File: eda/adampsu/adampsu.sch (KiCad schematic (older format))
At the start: 39 parts, among them J1 Barrel_Jack_Switch, J2 Conn_2Rows-09Pins, J3 DB9_Female, Q1 BUK7880-55A_CUX, SW1 30V 300mA Latching Switch, U1 LM27761

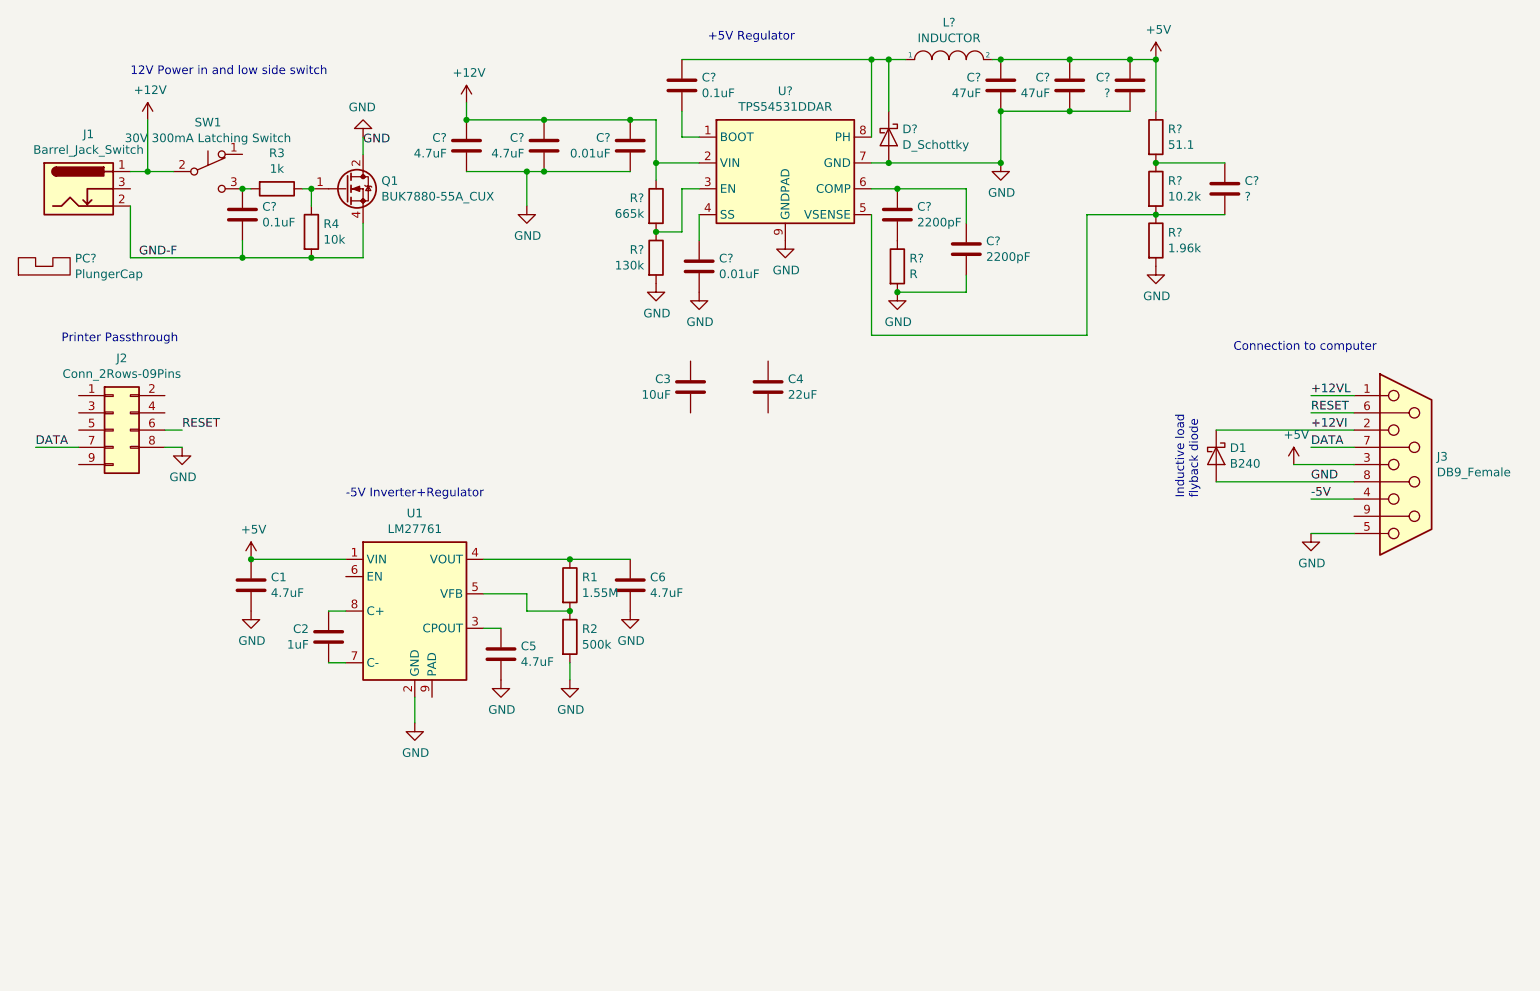
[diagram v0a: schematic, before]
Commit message: Final parts selection finished
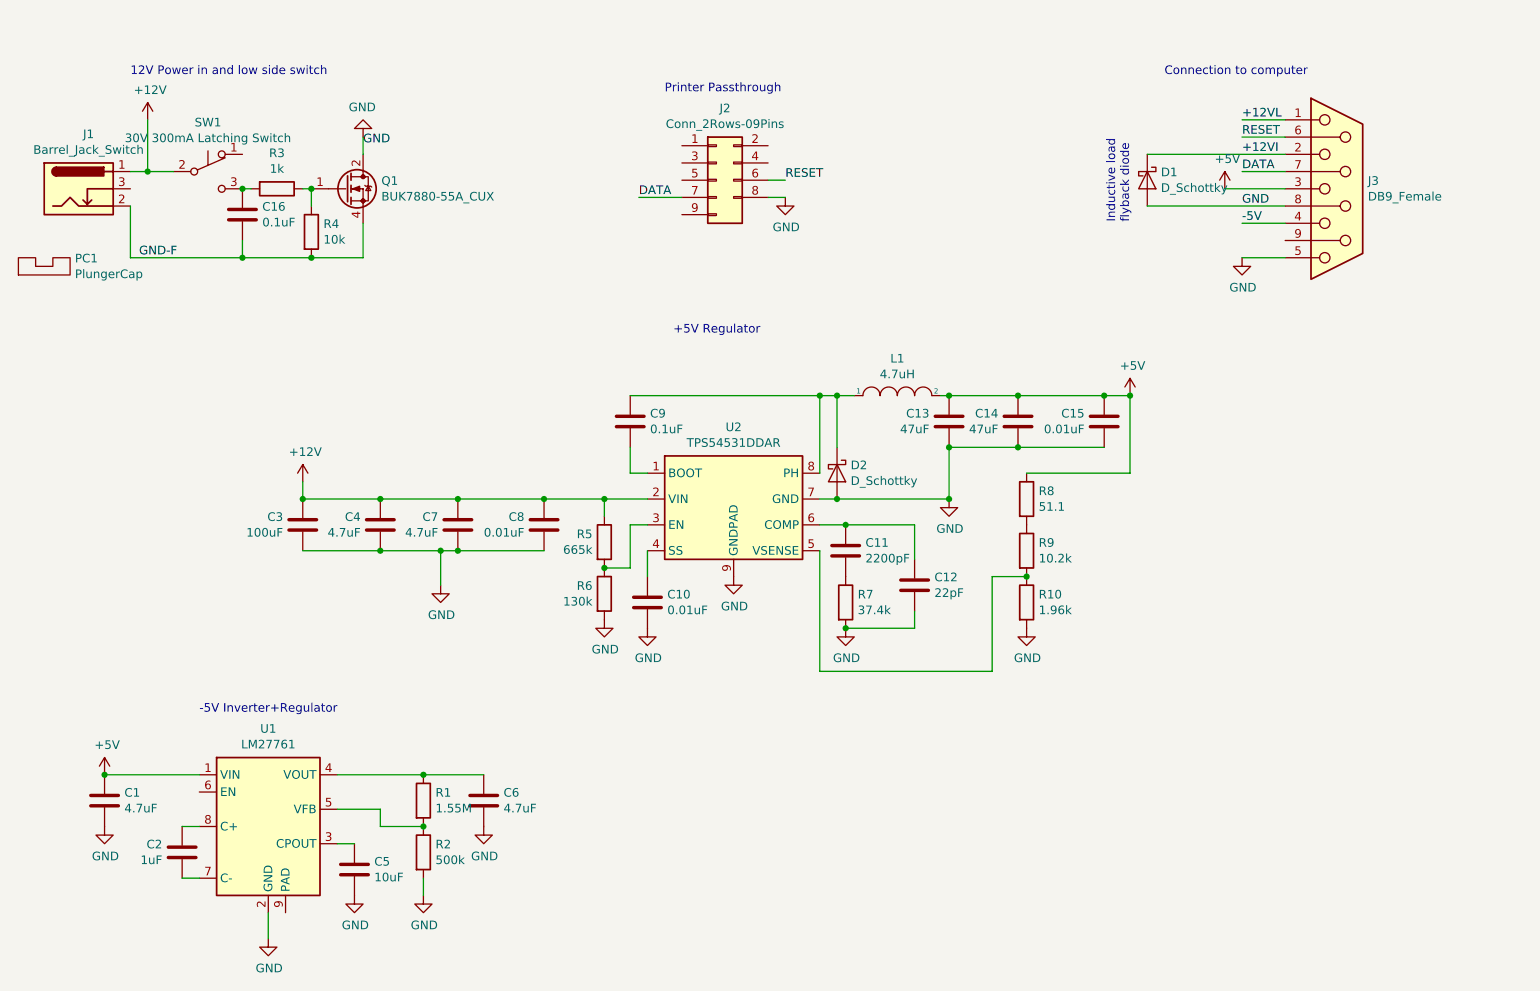
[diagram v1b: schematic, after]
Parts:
- removed C3: 10uF, Capacitor_SMD:C_1206_3216Metric_Pad1.42x1.75mm_HandSolder, symbol adampsu-rescue:C-Device
- removed C? (x2): ?, symbol adampsu-rescue:C-Device
- added C15: 0.01uF, Capacitor_SMD:C_0603_1608Metric_Pad1.05x0.95mm_HandSolder, symbol adampsu-rescue:C-Device
- C1, C6: footprint Capacitor_SMD:C_0603_1608Metric_Pad1.05x0.95mm_HandSolder -> Capacitor_SMD:C_1206_3216Metric_Pad1.42x1.75mm_HandSolder; dk 1276-2087-1-ND -> GRM32ER71H475KA88L; maxV (none) -> 50; mfr CL10B475KQ8NQNC -> UMK316AB7475KL-T; rating (none) -> XR7
- C10, C8: renamed from C?; dk (none) -> 399-7842-1-ND; mfr (none) -> C0603C103M5RACTU; rating (none) -> XR7
- C11: renamed from C?; footprint (none) -> Capacitor_SMD:C_0603_1608Metric_Pad1.05x0.95mm_HandSolder; dk (none) -> 399-17586-1-ND; maxV (none) -> 50; mfr (none) -> C0603C222K5RAC7411; rating (none) -> XR7
- C12: renamed from C?; value 2200pF -> 22pF; footprint (none) -> Capacitor_SMD:C_0603_1608Metric_Pad1.05x0.95mm_HandSolder; dk (none) -> 478-6204-1-ND; maxV (none) -> 50; mfr (none) -> 06035C220JAT2A; rating (none) -> XR7
- C13, C14: renamed from C?; footprint (none) -> Capacitor_SMD:C_1210_3225Metric_Pad1.42x2.65mm_HandSolder; dk (none) -> 587-5922-1-ND; maxV (none) -> 10+; mfr (none) -> LMK325B7476MM-PR; rating (none) -> XR7
- C16: renamed from C?; footprint (none) -> Capacitor_SMD:C_0603_1608Metric_Pad1.05x0.95mm_HandSolder; dk (none) -> 1276-1012-2-ND; maxV (none) -> 25; mfr (none) -> CL10F104ZB8NNNC; rating (none) -> XR7
- C2: dk 1276-6524-1-ND -> 399-11133-1-ND; maxV (none) -> 10; mfr CL10B105MO8NNWC -> C0603C105K8RACTU; rating (none) -> XR7
- C3: renamed from C?; value 4.7uF -> 100uF; footprint Capacitor_SMD:C_0603_1608Metric_Pad1.05x0.95mm_HandSolder -> Capacitor_THT:CP_Radial_D8.0mm_P3.50mm; dk 1276-2087-1-ND -> 1189-1659-1-ND; maxV (none) -> 50; mfr CL10B475KQ8NQNC -> 50YXJ100MT78X11.5; rating (none) -> XR7
- C4: value 22uF -> 4.7uF; dk 1276-2769-1-ND -> GRM32ER71H475KA88L; maxV (none) -> 50; mfr CL31B226KPHNNNE -> UMK316AB7475KL-T; rating (none) -> XR7
- C5: value 4.7uF -> 10uF; footprint Capacitor_SMD:C_0603_1608Metric_Pad1.05x0.95mm_HandSolder -> Capacitor_SMD:C_0805_2012Metric_Pad1.15x1.40mm_HandSolder; dk 1276-2087-1-ND -> 490-14381-1-ND; maxV (none) -> 10+; mfr CL10B475KQ8NQNC -> GRM21BR71A106KA73K; rating (none) -> XR7
- C7: renamed from C?; footprint Capacitor_SMD:C_0603_1608Metric_Pad1.05x0.95mm_HandSolder -> Capacitor_SMD:C_1206_3216Metric_Pad1.42x1.75mm_HandSolder; dk 1276-2087-1-ND -> GRM32ER71H475KA88L; maxV (none) -> 50; mfr CL10B475KQ8NQNC -> UMK316AB7475KL-T; rating (none) -> XR7
- C9: renamed from C?; footprint (none) -> adampsu:C_0508_1220Metric_Pad1.40x1.15mm_HandSolder; dk (none) -> 490-4346-1-ND; maxV (none) -> 25; mfr (none) -> LLL216R71E104MA01L; rating (none) -> XR7
- D1: value B240 -> D_Schottky; footprint Diode_SMD:D_SMA-SMB_Universal_Handsoldering -> Diode_SMD:D_SMC_Handsoldering; dk B240A-E3/61TGICT-ND -> 641-1126-1-ND; maxV (none) -> 40; mfr B240A-E3/61T -> CDBC540-G
- D2: renamed from D?; footprint (none) -> Diode_SMD:D_SMC_Handsoldering; dk (none) -> 641-1126-1-ND; maxV (none) -> 40; mfr (none) -> CDBC540-G
- J2: dk (none) -> 1849-1002-ND; mfr (none) -> PR20205VBDN
- L1: renamed from L?; value INDUCTOR -> 4.7uH; footprint (none) -> adampsu:L_11.5x10.3_H4.8; dk (none) -> 553-3001-1-ND; mfr (none) -> PA4342.472NLT; rating (none) -> 15.5mOhm
- R10: renamed from R?; footprint (none) -> Resistor_SMD:R_0603_1608Metric_Pad1.05x0.95mm_HandSolder; dk (none) -> 311-1.96KHRCT-ND; mfr (none) -> RC0603FR-071K96L
- R5: renamed from R?; footprint (none) -> Resistor_SMD:R_0603_1608Metric_Pad1.05x0.95mm_HandSolder; dk (none) -> 311-665KHRCT-ND; mfr (none) -> RES SMD 665K OHM 1% 1/10W 0603
- R6: renamed from R?; footprint (none) -> Resistor_SMD:R_0603_1608Metric_Pad1.05x0.95mm_HandSolder; dk (none) -> 2019-RK73B1JTTD134JCT-ND; mfr (none) -> RK73B1JTTD134J
- R7: renamed from R?; value R -> 37.4k; footprint (none) -> Resistor_SMD:R_0603_1608Metric_Pad1.05x0.95mm_HandSolder; dk (none) -> 311-37.4KHRCT-ND; mfr (none) -> RC0603FR-0737K4L
- R8: renamed from R?; footprint (none) -> Resistor_SMD:R_0603_1608Metric_Pad1.05x0.95mm_HandSolder; dk (none) -> 311-51.1HRCT-ND; mfr (none) -> RC0603FR-0751R1L
- R9: renamed from R?; footprint (none) -> Resistor_SMD:R_0603_1608Metric_Pad1.05x0.95mm_HandSolder; dk (none) -> RMCF0603FT10K2CT-ND; mfr (none) -> RMCF0603FT10K2
- U2: renamed from U?; dk (none) -> 296-40801-2-ND; mfr (none) -> TPS54531DDAR
- gave numbers to parts that had none: 1
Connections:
- net +12V: now also C4.1
- net +5V: now also C15.1
- net GND: now also C4.2, C15.2
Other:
- moved on the sheet: C1, C10, C11, C12, C13, C14, C2, C3, C5, C6, C7, C8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
